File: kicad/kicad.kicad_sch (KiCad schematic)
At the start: 128 parts, among them SW1 SW_Push, SW10 SW_Push, SW11 SW_Push, SW12 SW_Push, SW13 SW_Push, SW14 SW_Push, SW15 SW_Push, SW16 SW_Push, SW17 SW_Push, SW18 SW_Push, SW19 SW_Push, SW2 SW_Push, SW20 SW_Push, SW21 SW_Push, SW22 SW_Push, SW23 SW_Push, SW24 SW_Push, SW25 SW_Push, SW26 SW_Push, SW27 SW_Push, SW28 SW_Push, SW29 SW_Push, SW3 SW_Push, SW30 SW_Push, SW31 SW_Push, SW32 SW_Push, SW33 SW_Push, SW34 SW_Push, SW35 SW_Push, SW36 SW_Push, SW37 SW_Push, SW38 SW_Push, SW39 SW_Push, SW4 SW_Push, SW40 SW_Push, SW41 SW_Push, SW42 SW_Push, SW43 SW_Push, SW44 SW_Push, SW45 SW_Push, SW46 SW_Push, SW47 SW_Push, SW48 SW_Push, SW49 SW_Push, SW5 SW_Push, SW50 SW_Push, SW51 SW_Push, SW52 SW_Push, SW53 SW_Push, SW54 SW_Push, SW55 SW_Push, SW56 SW_Push, SW57 SW_Push, SW58 SW_Push, SW59 SW_Push, SW6 SW_Push, SW60 SW_Push, SW61 SW_Push, SW7 SW_Push, SW8 SW_Push, SW9 SW_Push

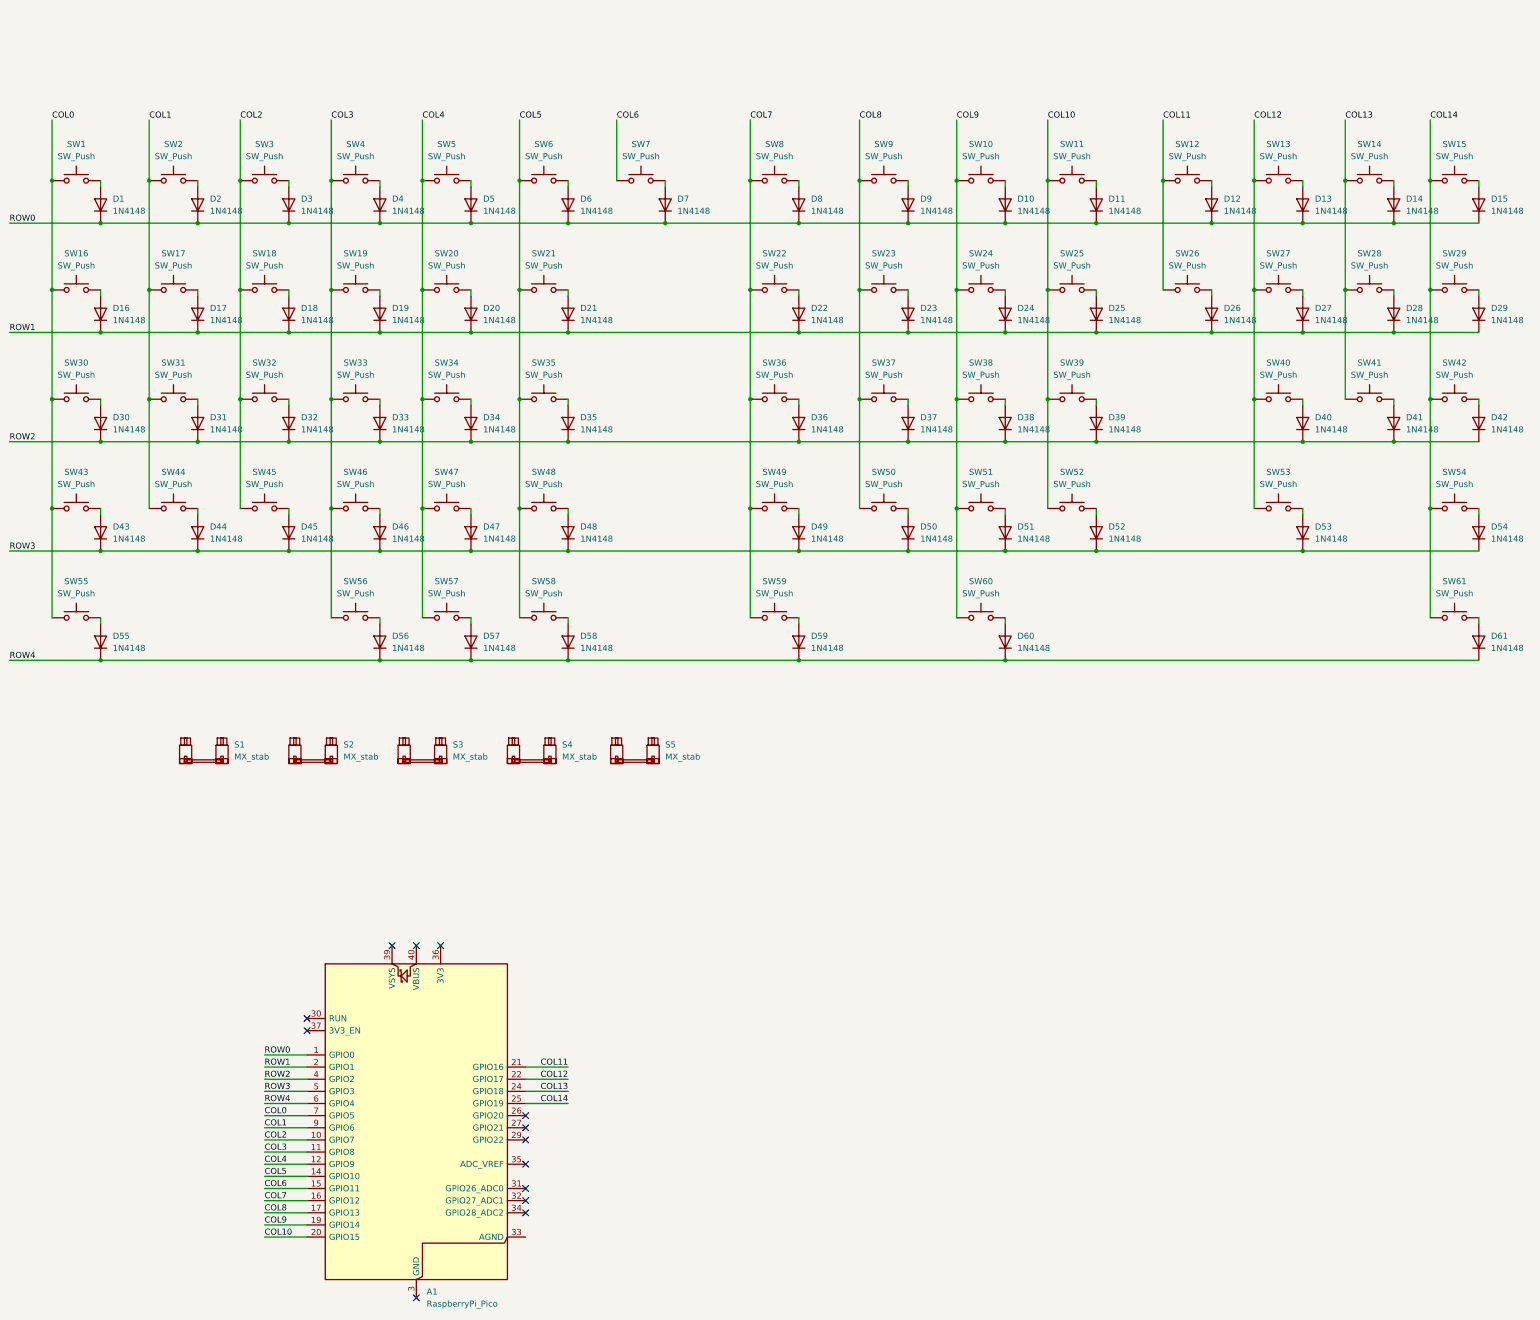
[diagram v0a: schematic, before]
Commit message: restarting again aaa
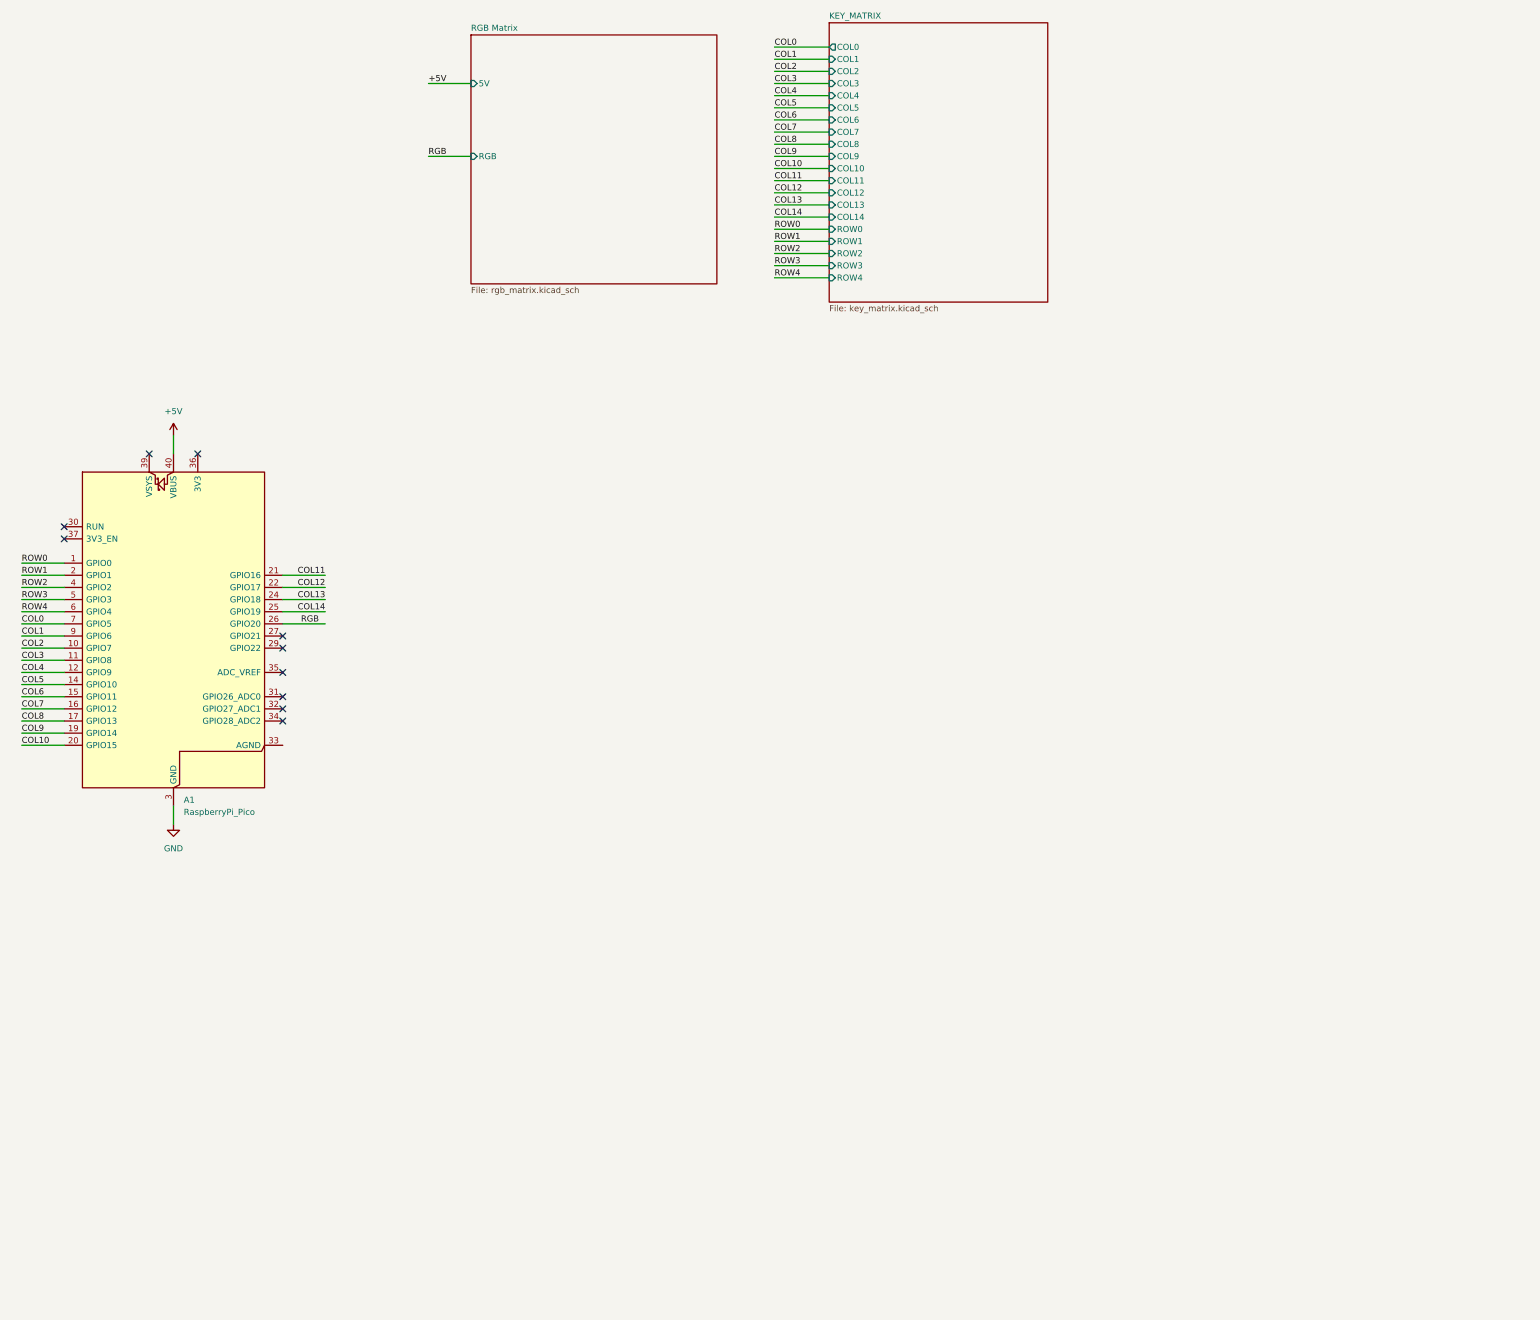
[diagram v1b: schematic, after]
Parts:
- removed D1, D10, D11, D12, D13, D14, D15, D16, D17, D18, D19, D2, D20, D21, D22, D23, D24, D25, D26, D27, D28, D29, D3, D30, D31, D32, D33, D34, D35, D36, D37, D38, D39, D4, D40, D41, D42, D43, D44, D45, D46, D47, D48, D49, D5, D50, D51, D52, D53, D54, D55, D56, D57, D58, D59, D6, D60, D61, D7, D8, D9: 1N4148, Diode_THT:D_DO-35_SOD27_P7.62mm_Horizontal, symbol Diode:1N4148
- removed S1: MX_stab, PCM_marbastlib-mx:STAB_MX_3u, symbol PCM_marbastlib-mx:MX_stab
- removed S2: MX_stab, PCM_marbastlib-mx:STAB_MX_2u, symbol PCM_marbastlib-mx:MX_stab
- removed S3, S4, S5: MX_stab, PCM_marbastlib-mx:STAB_MX_2.25u, symbol PCM_marbastlib-mx:MX_stab
- removed SW1, SW10, SW11, SW12, SW13, SW14, SW15, SW16, SW17, SW18, SW19, SW2, SW20, SW21, SW22, SW23, SW24, SW25, SW26, SW27, SW28, SW29, SW3, SW30, SW31, SW32, SW33, SW34, SW35, SW36, SW37, SW38, SW39, SW4, SW40, SW41, SW42, SW43, SW44, SW45, SW46, SW47, SW48, SW49, SW5, SW50, SW51, SW52, SW53, SW54, SW55, SW56, SW57, SW58, SW59, SW6, SW60, SW61, SW7, SW8, SW9: SW_Push, PCM_marbastlib-mx:SW_MX_1u, symbol Switch:SW_Push
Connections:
- net GND: now reaches A1.13 (GND), A1.18 (GND), A1.23 (GND), A1.28 (GND), A1.3 (GND), A1.38 (GND), A1.8 (GND)
- net RGB: now reaches A1.26 (GPIO20)
- net +5V: now reaches A1.40 (VBUS)
- no-connect marks 13 -> 10
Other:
- added sheet KEY_MATRIX (key_matrix.kicad_sch)
- added sheet RGB Matrix (rgb_matrix.kicad_sch)
- moved on the sheet: A1
